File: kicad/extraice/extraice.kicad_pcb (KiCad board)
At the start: 2 copper layers, 77 x 57.8 mm, 73 parts, among them J1 Conn_01x02, J10 Conn_01x02, J3 EncSide, J4 MainSide, J5 Conn_01x05, J6 EncSide, J7 MainSide, J8 Conn_01x02, J9 Conn_01x02, Q1 L-31ROPT1C, Q2 L-31ROPT1C, Q3 L-31ROPT1C, Q4 L-31ROPT1C, SW1 PCM12SMTR, SW2 B3U-1000P, U1 DG2034EDN, U10 DRV8837C, U11 DRV8837C, U12 AS5047D, U2 BCR421, U3 MUN12AD01-SG, U4 MB85RC64TA, U5 LSM6DSR, U6 XC6221B302GR, U7 ESP32-S3-FN8, U8 AS5047D, U9 DRV8837C, X1 830108208709

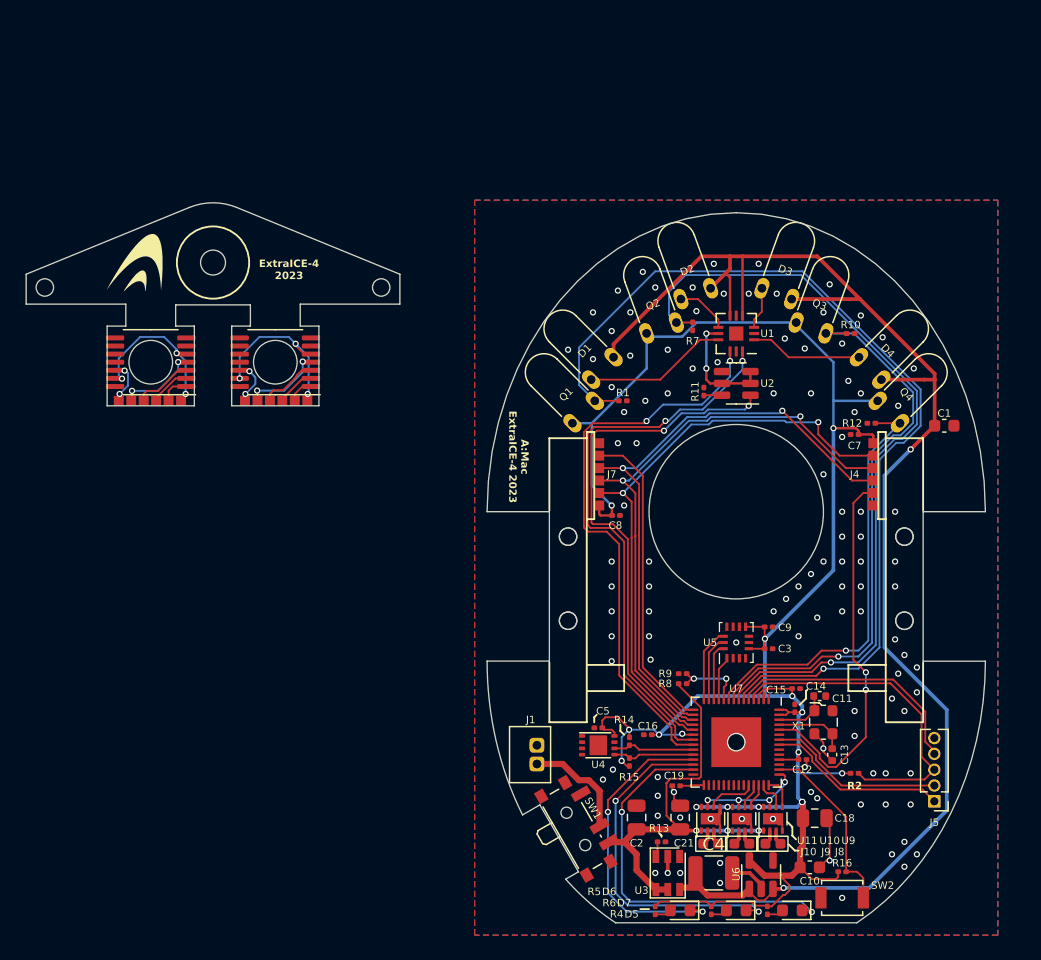
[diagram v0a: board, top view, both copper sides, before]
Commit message: Artwork for 4A completed
Need to check details.

Signed-off-by: Kazuki Iida <elkel53930@gmail.com>
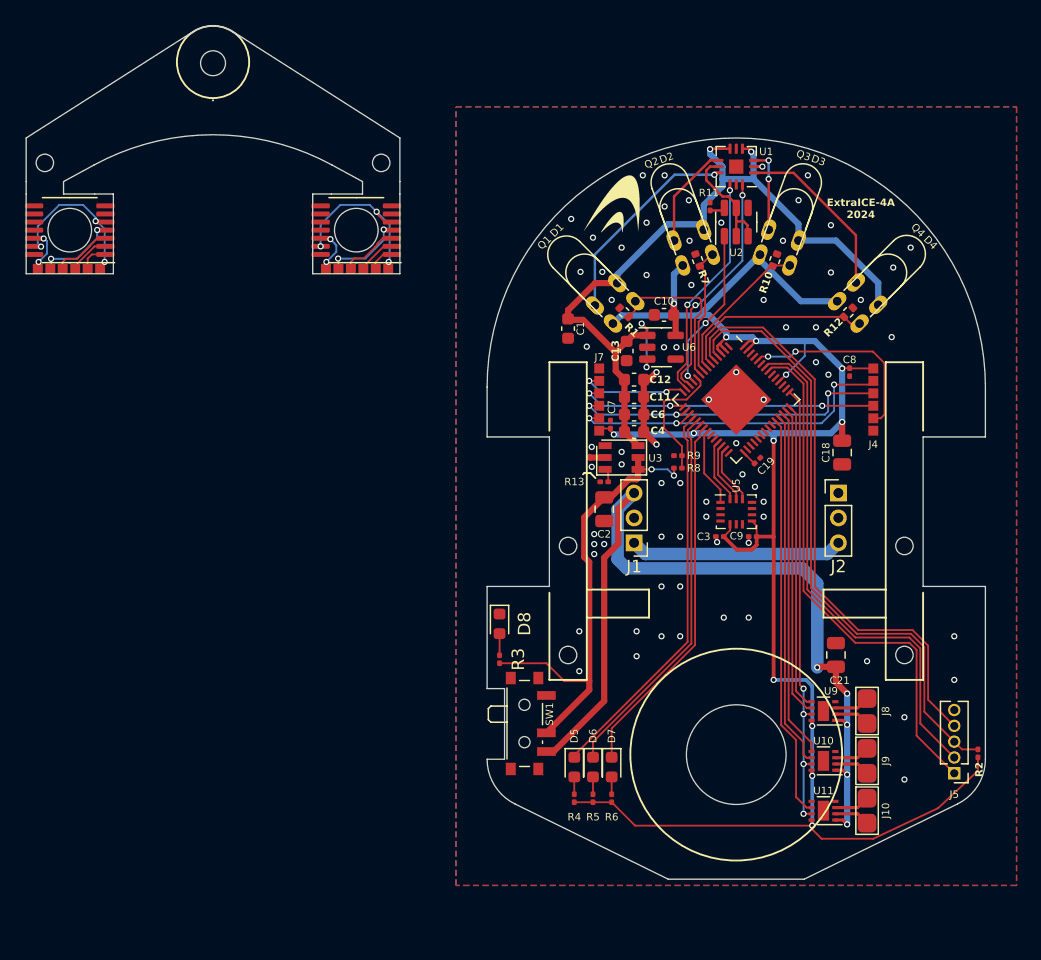
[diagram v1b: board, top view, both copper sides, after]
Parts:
- removed C14, C15, C16, C5: 0603 50V 0.1uF, Capacitor_SMD:C_0201_0603Metric
- removed R14, R15, R16: 0603 10k, Resistor_SMD:R_0201_0603Metric
- removed SW2: B3U-1000P, Button_Switch_SMD:SW_SPST_B3U-1000P
- removed U4: MB85RC64TA, Library:LCC-8P-M04
- removed X1: 830108208709, Oscillator:Oscillator_SMD_ECS_2520MV-xxx-xx-4Pin_2.5x2.0mm
- added C6: 1608 10V 4.7uF, Capacitor_SMD:C_0603_1608Metric, F.Cu at (131.8, 92.2)
- added D8: 1608 R LED, LED_SMD:LED_0603_1608Metric, F.Cu at (121.0, 109.0)
- added J2: Conn_01x03, Connector_PinHeader_2.00mm:PinHeader_1x03_P2.00mm_Vertical, F.Cu at (148.2, 98.5)
- added R3: 0603 10k, Resistor_SMD:R_0201_0603Metric, F.Cu at (121.0, 111.8)
- C11, C13: value 1005 N/M -> 1608 10V 4.7uF; footprint Capacitor_SMD:C_0402_1005Metric -> Capacitor_SMD:C_0603_1608Metric
- C12: value 0603 50V 0.1uF -> 1608 10V 4.7uF; footprint Capacitor_SMD:C_0201_0603Metric -> Capacitor_SMD:C_0603_1608Metric
- C4: value 3225 25V 22uF -> 1608 10V 4.7uF; footprint Capacitor_SMD:C_1210_3225Metric -> Capacitor_SMD:C_0603_1608Metric
- J1: value Conn_01x02 -> Conn_01x03; footprint Micromouse:B2B-ZH -> Connector_PinHeader_2.00mm:PinHeader_1x03_P2.00mm_Vertical
- R1, R10, R12, R7: value 0603 470 1% -> 1005 470 1%; footprint Resistor_SMD:R_0201_0603Metric -> Resistor_SMD:R_0402_1005Metric
- U7: value ESP32-S3-FN8 -> ESP32-S3-PICO-1-N8R2
- moved C10 45.9 mm to (134.2, 84.2), turned to 180 degrees
- moved U6 43.1 mm to (134.0, 86.8), turned to 0 degrees
- moved G*** 38.6 mm to (129.8, 75.2)
- moved C13 36.4 mm to (131.2, 87.1), turned to 90 degrees
- moved C4 36.0 mm to (131.8, 93.6), turned to 180 degrees
- moved U3 33.6 mm to (130.8, 95.7), turned to 0 degrees
- moved C12 33.4 mm to (131.8, 89.4), turned to 180 degrees
- moved C1 31.2 mm to (126.5, 85.3), turned to -90 degrees
- moved C18 29.4 mm to (148.5, 95.2), turned to -90 degrees
- moved R13 29.3 mm to (129.4, 97.6), turned to 0 degrees
- moved H3 28.6 mm to (126.5, 111.5)
- moved C11 28.2 mm to (131.8, 90.8), turned to 180 degrees
- moved H2 27.7 mm to (153.5, 102.8)
- moved U7 27.5 mm to (140.0, 91.0), turned to -45 degrees
- moved C19 26.9 mm to (141.7, 95.9), turned to 45 degrees
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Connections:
- C11 pad 1: Net-(U7-XTAL_P) -> GND
- C11 pad 2: GND -> +3.3V
- C12 pad 1: +3V0 -> GND
- C12 pad 2: GND -> +3.3V
- C13 pad 1: Net-(U7-XTAL_N) -> GND
- C13 pad 2: GND -> +3.3V
- C21 pad 1: +BATT -> /V_MOT
- C4 pad 1: +3.3V -> GND
- C4 pad 2: GND -> +3.3V
- D5 pad 1: /LED_LEFT_R -> /LED_R
- D6 pad 1: /LED_RIGHT_G -> /LED_G
- D7 pad 1: /LED_FRONT_B -> /LED_B
- J1 pad 1: GND -> Net-(J1-Pin_1)
- J1 pad 2: Net-(J1-Pin_2) -> unconnected-(J1-Pin_2-Pad2)
- SW1 pad 2: Net-(J1-Pin_2) -> +BATT
- SW1 pad 3: +BATT -> /V_MOT
- U10 pad 1: +BATT -> /V_MOT
- U11 pad 1: +BATT -> /V_MOT
- U7 pad 11: /SPI2_MISO -> /SEN_LED_ENA
- U7 pad 12: /SPI2_MOSI -> /LED_SEL0
- U7 pad 13: /SPI2_SCK -> /LED_SEL1
- U7 pad 14: /CS_IMU -> /CS_ENC_L
- U7 pad 15: /CS_ENC_L -> /SPI1_SCK
- U7 pad 16: /SPI1_SCK -> /SPI1_MISO
- U7 pad 17: /SPI1_MISO -> /SPI1_MOSI
- U7 pad 18: /SPI1_MOSI -> /LED_R
- U7 pad 19: /SEN_LED_ENA -> /LED_G
- U7 pad 21: /LED_SEL0 -> /LED_B
- U7 pad 22: /LED_SEL1 -> /SPI2_MISO
- U7 pad 23: /SCL -> unconnected-(U7-GPIO17-Pad23)
- U7 pad 24: /SDA -> unconnected-(U7-GPIO18-Pad24)
- U7 pad 25: /LED_RIGHT_G -> /SPI2_MOSI
- U7 pad 26: /LED_FRONT_B -> /SPI2_SCK
- U7 pad 27: /LED_LEFT_R -> /CS_IMU
- U7 pad 44: Net-(U7-MTCK) -> unconnected-(U7-MTCK-Pad44)
- U7 pad 53: Net-(U7-XTAL_N) -> unconnected-(U7-XTAL_N-Pad53)
- U7 pad 54: Net-(U7-XTAL_P) -> unconnected-(U7-XTAL_P-Pad54)
- U7 pad 6: /SEN_LS -> /SEN_RS
- U7 pad 7: /SEN_LF -> /SEN_RF
- U7 pad 8: /SEN_RF -> /SEN_LF
- U7 pad 9: /SEN_RS -> /SEN_LS
- U9 pad 1: +BATT -> /V_MOT
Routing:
- net /V_MOT: track 0.00 -> 71.4 mm, vias 0 -> 5
- net /SEN_LS: track 75.9 -> 13.4 mm, vias 1 -> 0
- net /SEN_LF: track 63.5 -> 10.4 mm, vias 1 -> 0
- net +3.3V: track 119.4 -> 68.3 mm, vias 2 -> 4
- net /SEN_RF: track 45.7 -> 12.1 mm, vias 1 -> 0
- net /LED_R: track 0.00 -> 31.5 mm
- net /LED_LEFT_R: track 30.8 -> 0.00 mm, vias 2 -> 0
- net /LED_G: track 0.00 -> 30.7 mm
- net /SEN_LED_ENA: track 42.9 -> 13.1 mm
- net /LED_B: track 0.00 -> 29.5 mm
- net /PWM_V: track 3.99 -> 32.5 mm
- net /LED_FRONT_B: track 28.0 -> 0.00 mm, vias 2 -> 0
- net /TXD: track 14.6 -> 42.3 mm
- net /GPIO0: track 19.8 -> 47.4 mm
- net /LED_SEL1: track 46.0 -> 18.4 mm
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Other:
- board size 77 x 57.8 mm -> 77 x 68.5 mm
- board text added: "ExtraICE-4A 2024"
- board text removed: "A:Mac ExtraICE-4 2023"
- board text removed: "ExtraICE-4 2023"
